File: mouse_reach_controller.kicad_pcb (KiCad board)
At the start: 2 copper layers, 158.8 x 57.2 mm, 115 parts, among them J1 AUDIO_JACK_3.5MM, P1 HEADER_02X05_LATCH, P2 HEADER_02X05_LATCH, P3 HEADER_02X05_LATCH, P4 PWR_JACK_2.1x5.5_SMD_RA, P5 BNC_DOUBLE_RA, P6 BNC_DOUBLE_RA, P7 BNC_DOUBLE_RA, T1 TERM_BLK_HDR_2POS_90DEG_0.2IN, T2 TERM_BLK_HDR_4POS_90DEG_0.2IN, U1 TMC429, U10 SGTL5000, U11 RT9076-15GV, U12 74LVC1G125GS, U13 74LVC1G125GS, U14 TMC424, U15 74LVC1G125GS, U16 74LVC1G125GS, U17 74LVC1G125GS, U18 74LVC1G125GS, U19 74LVC1G125GS, U2 SN65LVDM050QDRQ1, U20 74LVC1G125GS, U3 74LVC1G125GS, U4 SN65LVDM050QDRQ1, U5 74LVC1G125GS, U6 SN65LVDM050QDRQ1, U7 74LVC1G125GS, U8 ZXMS6006SG, U9 RT9076-15GV

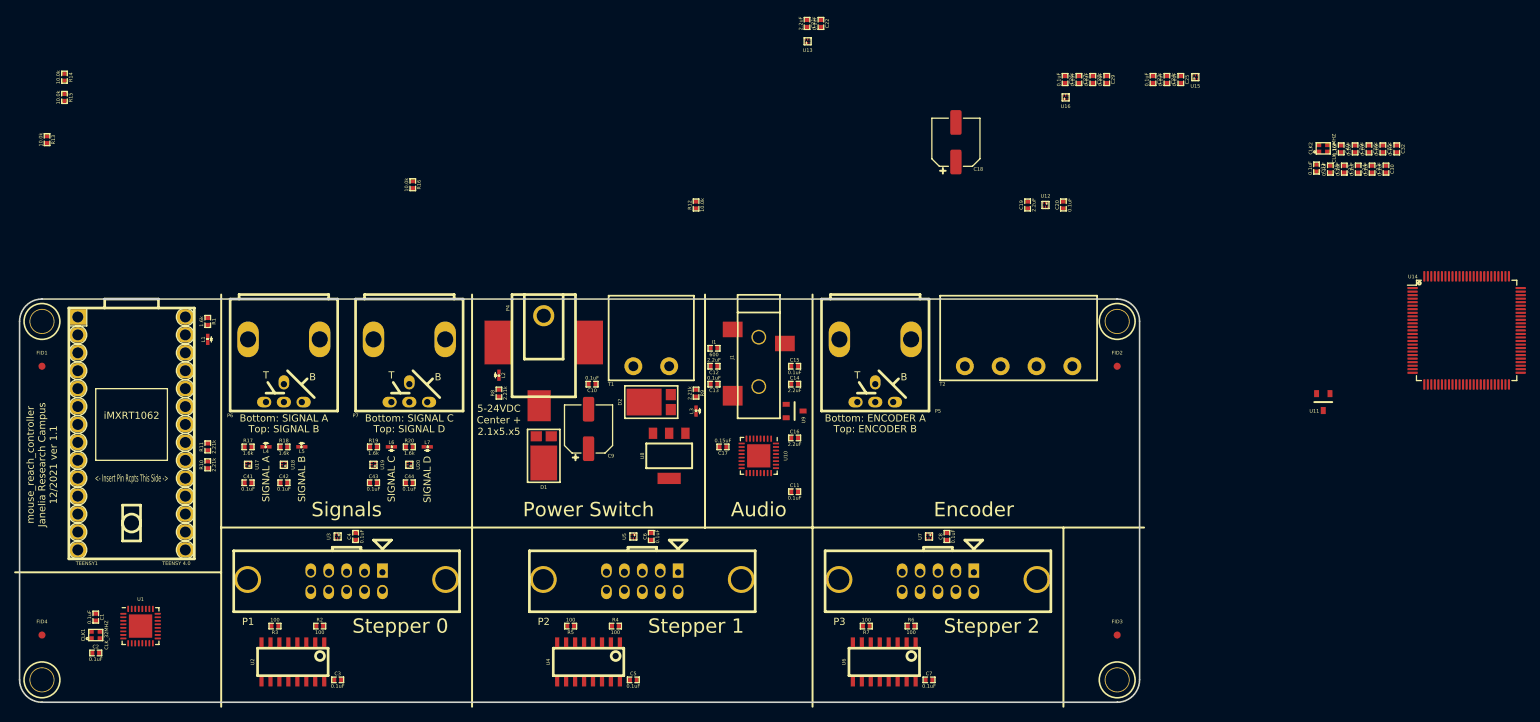
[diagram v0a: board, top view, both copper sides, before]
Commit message: Route board
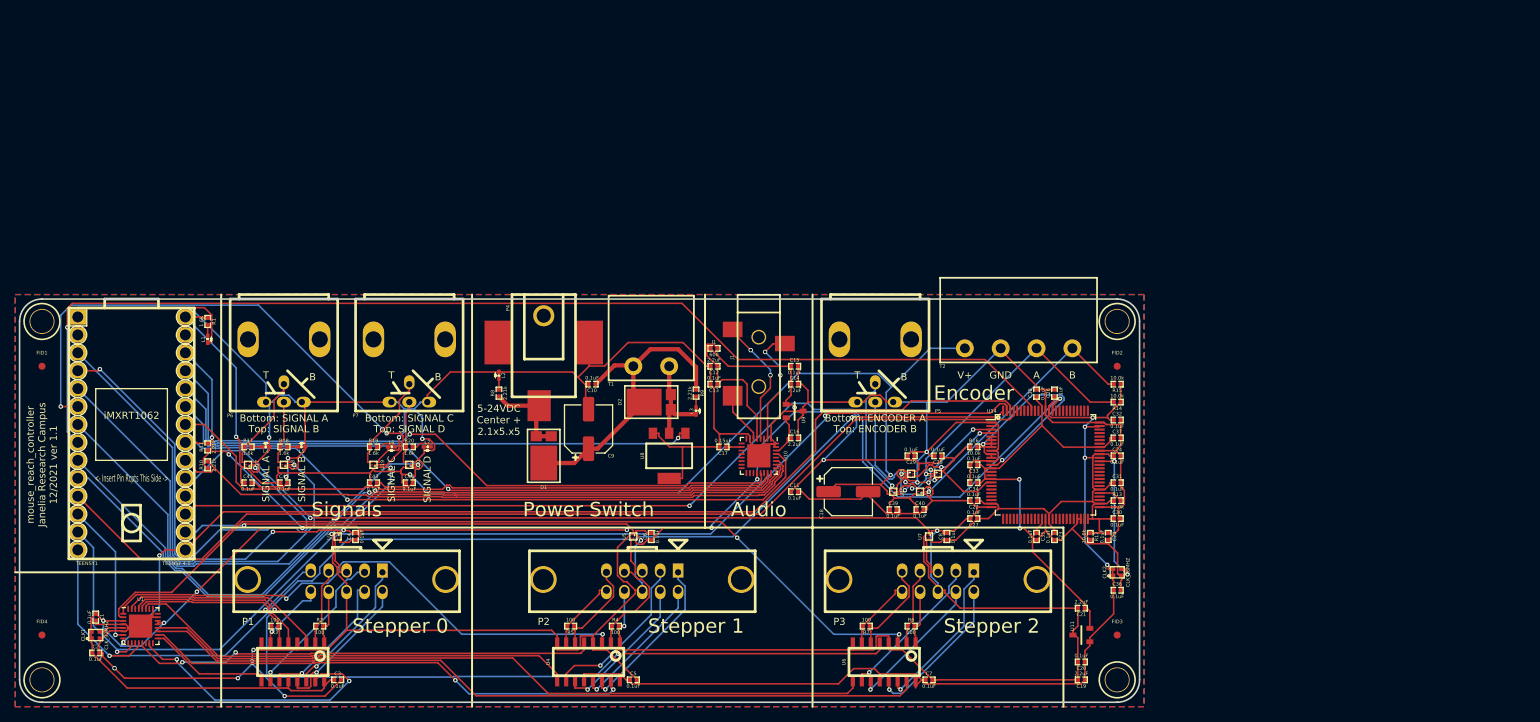
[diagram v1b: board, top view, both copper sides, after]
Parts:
- moved R13 160.1 mm to (224.8, 80.0), turned to 90 degrees
- moved R14 156.2 mm to (224.8, 66.0), turned to 270 degrees
- moved R15 154.6 mm to (224.8, 63.5), turned to 270 degrees
- moved C21 91.5 mm to (219.7, 95.2), turned to 270 degrees
- moved R16 87.8 mm to (204.5, 72.4), turned to 90 degrees
- moved C39 83.1 mm to (193.0, 81.3), turned to 90 degrees
- moved C40 78.6 mm to (196.8, 81.3), turned to 90 degrees
- moved C35 73.7 mm to (213.4, 85.1)
- moved R12 73.0 mm to (221.0, 85.1), turned to 0 degrees
- moved U15 72.7 mm to (193.0, 78.7), turned to 90 degrees
- moved C36 72.0 mm to (224.8, 92.7), turned to 90 degrees
- moved C22 71.0 mm to (204.5, 80.0), turned to 270 degrees
- moved C34 70.3 mm to (204.5, 77.5), turned to 270 degrees
- moved C33 70.3 mm to (204.5, 74.9), turned to 270 degrees
- moved C19 67.7 mm to (219.7, 105.4), turned to 270 degrees
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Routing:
- net /GND: track 0.00 -> 798.4 mm, vias 0 -> 19
- net /VDD: track 0.00 -> 505.7 mm, vias 0 -> 15
- net /VCC: track 0.00 -> 186.9 mm, vias 0 -> 3
- net /MOSI: track 0.00 -> 163.8 mm, vias 0 -> 2
- net /MISO: track 0.00 -> 163.7 mm, vias 0 -> 2
- net /~ENCODER_RESET: track 0.00 -> 163.3 mm, vias 0 -> 1
- net /SCK: track 0.00 -> 148.2 mm, vias 0 -> 2
- net /ENCODER_INVERT: track 0.00 -> 147.4 mm, vias 0 -> 2
- net /~ENCODER_CS: track 0.00 -> 145.5 mm
- net /stepper_controller/REF_2: track 0.00 -> 125.4 mm, vias 0 -> 2
- net /stepper_controller/REFR_2: track 0.00 -> 120.0 mm, vias 0 -> 2
- net /I2S_DIN: track 0.00 -> 117.6 mm, vias 0 -> 1
- net /I2S_DOUT: track 0.00 -> 115.0 mm, vias 0 -> 1
- net /UART_2: track 0.00 -> 112.2 mm, vias 0 -> 1
- net /stepper_controller/STEP_2: track 0.00 -> 111.5 mm
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- added copper zone on B.Cu, net /GND
- added copper zone on F.Cu, net /GND
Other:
- net class THICKPOWER: clearance 0.2032 -> 0.1016; trace_width 1.524 -> 0.6096; via_dia 1.524 -> 0.635; via_drill 0.635 -> 0.4064
- net class THICKSIGNAL: clearance 0.2032 -> 0.1016; via_dia 0.9144 -> 0.635; via_drill 0.635 -> 0.4064
- board text added: "A"
- board text added: "B"
- board text added: "GND"
- board text added: "V+"
